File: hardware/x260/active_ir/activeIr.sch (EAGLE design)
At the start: 8 parts, among them Q1 MOSFET-N

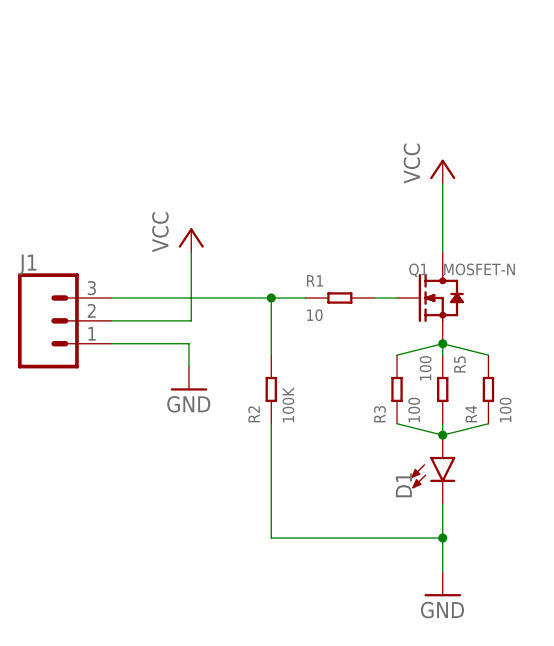
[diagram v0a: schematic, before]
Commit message: Initial simulation implementation
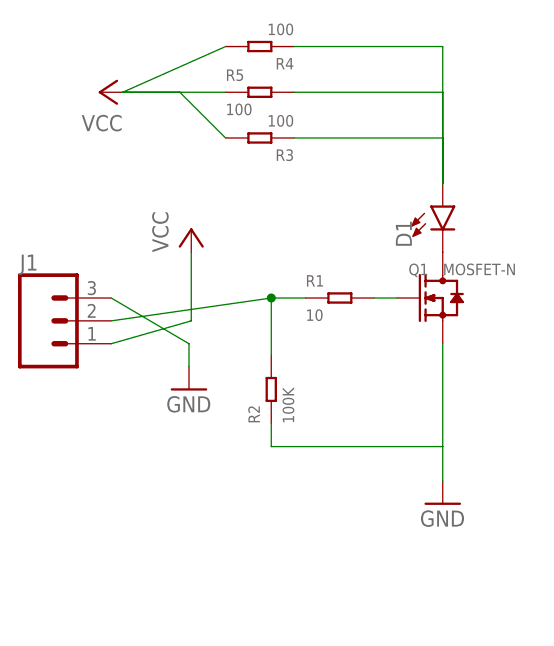
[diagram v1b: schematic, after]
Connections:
- net GND: now also J1.3, Q1.S; no longer D1.C, J1.1
- net N$1: now also D1.C, Q1.D; no longer Q1.S, R3.2, R4.2, R5.1
- net SIGNAL: now also J1.2; no longer J1.3
- net VCC: now also J1.1, R3.2, R4.2, R5.1; no longer J1.2, Q1.D
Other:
- moved on the sheet: D1, R3, R4, R5
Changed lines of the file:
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@@
 <instances>
 <instance part="Q1" gate="Q" x="53.34" y="45.72"/>
-<instance part="P+1" gate="VCC" x="53.34" y="60.96"/>
-<instance part="GND1" gate="1" x="53.34" y="12.7"/>
-<instance part="D1" gate="G$1" x="53.34" y="27.94"/>
+<instance part="P+1" gate="VCC" x="15.24" y="68.58" rot="R90"/>
+<instance part="GND1" gate="1" x="53.34" y="22.86"/>
+<instance part="D1" gate="G$1" x="53.34" y="55.88"/>
 <instance part="R2" gate="R" x="34.29" y="35.56" rot="R90"/>
 <instance part="R1" gate="R" x="41.91" y="45.72"/>
-<instance part="R3" gate="R" x="48.26" y="35.56" rot="R90"/>
+<instance part="R3" gate="R" x="33.02" y="63.5" rot="R180"/>
 <instance part="J1" gate="J$1" x="8.89" y="43.18"/>
 <instance part="P+2" gate="VCC" x="25.4" y="53.34"/>
 <instance part="GND2" gate="1" x="25.146" y="35.56"/>
-<instance part="R4" gate="R" x="58.42" y="35.56" rot="R90"/>
-<instance part="R5" gate="R" x="53.34" y="35.56" rot="R270"/>
+<instance part="R4" gate="R" x="33.02" y="73.66" rot="R180"/>
+<instance part="R5" gate="R" x="33.02" y="68.58"/>
 </instances>
 <busses>
@@
 <net name="VCC" class="0">
 <segment>
-<pinref part="Q1" gate="Q" pin="D"/>
-<pinref part="P+1" gate="VCC" pin="VCC"/>
-<wire x1="53.34" y1="58.42" x2="53.34" y2="50.8" width="0.1524" layer="91"/>
+<pinref part="J1" gate="J$1" pin="1"/>
+<pinref part="P+2" gate="VCC" pin="VCC"/>
+<wire x1="25.4" y1="50.8" x2="25.4" y2="43.18" width="0.1524" layer="91"/>
+<wire x1="25.4" y1="43.18" x2="16.51" y2="40.64" width="0.1524" layer="91"/>
 </segment>
 <segment>
-<pinref part="J1" gate="J$1" pin="2"/>
-<pinref part="P+2" gate="VCC" pin="VCC"/>
-<wire x1="25.4" y1="50.8" x2="25.4" y2="43.18" width="0.1524" layer="91"/>
-<wire x1="25.4" y1="43.18" x2="16.51" y2="43.18" width="0.1524" layer="91"/>
+<pinref part="R4" gate="R" pin="2"/>
+<pinref part="P+1" gate="VCC" pin="VCC"/>
+<wire x1="29.21" y1="73.66" x2="17.78" y2="68.58" width="0.1524" layer="91"/>
+<pinref part="R5" gate="R" pin="1"/>
+<wire x1="29.21" y1="68.58" x2="17.78" y2="68.58" width="0.1524" layer="91"/>
+<pinref part="R3" gate="R" pin="2"/>
+<wire x1="29.21" y1="63.5" x2="24.13" y2="68.58" width="0.1524" layer="91"/>
+<wire x1="24.13" y1="68.58" x2="17.78" y2="68.58" width="0.1524" layer="91"/>
 </segment>
 </net>
 <net name="GND" class="0">
 <segment>
-<pinref part="D1" gate="G$1" pin="C"/>
 <pinref part="GND1" gate="1" pin="GND"/>
-<wire x1="53.34" y1="15.24" x2="53.34" y2="19.05" width="0.1524" layer="91"/>
 <pinref part="R2" gate="R" pin="1"/>
-<wire x1="53.34" y1="19.05" x2="53.34" y2="22.86" width="0.1524" layer="91"/>
-<wire x1="34.29" y1="31.75" x2="34.29" y2="19.05" width="0.1524" layer="91"/>
-<wire x1="34.29" y1="19.05" x2="53.34" y2="19.05" width="0.1524" layer="91"/>
-<junction x="53.34" y="19.05"/>
+<wire x1="53.34" y1="25.4" x2="53.34" y2="29.21" width="0.1524" layer="91"/>
+<wire x1="34.29" y1="31.75" x2="34.29" y2="29.21" width="0.1524" layer="91"/>
+<wire x1="34.29" y1="29.21" x2="53.34" y2="29.21" width="0.1524" layer="91"/>
+<pinref part="Q1" gate="Q" pin="S"/>
+<wire x1="53.34" y1="40.64" x2="53.34" y2="29.21" width="0.1524" layer="91"/>
 </segment>
 <segment>
-<pinref part="J1" gate="J$1" pin="1"/>
+<pinref part="J1" gate="J$1" pin="3"/>
 <pinref part="GND2" gate="1" pin="GND"/>
 <wire x1="25.146" y1="38.1" x2="25.146" y2="40.64" width="0.1524" layer="91"/>
-<wire x1="25.146" y1="40.64" x2="16.51" y2="40.64" width="0.1524" layer="91"/>
-</segment>
-</net>
-<net name="N$1" class="0">
-<segment>
-<pinref part="Q1" gate="Q" pin="S"/>
-<pinref part="R3" gate="R" pin="2"/>
-<wire x1="48.26" y1="39.37" x2="53.34" y2="40.64" width="0.1524" layer="91"/>
-<pinref part="R4" gate="R" pin="2"/>
-<wire x1="58.42" y1="39.37" x2="53.34" y2="40.64" width="0.1524" layer="91"/>
-<junction x="53.34" y="40.64"/>
-<pinref part="R5" gate="R" pin="1"/>
-<wire x1="53.34" y1="39.37" x2="53.34" y2="40.64" width="0.1524" layer="91"/>
+<wire x1="25.146" y1="40.64" x2="16.51" y2="45.72" width="0.1524" layer="91"/>
 </segment>
 </net>
@@
 <pinref part="R3" gate="R" pin="1"/>
 <pinref part="D1" gate="G$1" pin="A"/>
-<wire x1="53.34" y1="30.48" x2="48.26" y2="31.75" width="0.1524" layer="91"/>
+<wire x1="53.34" y1="58.42" x2="53.34" y2="63.5" width="0.1524" layer="91"/>
+<wire x1="53.34" y1="63.5" x2="36.83" y2="63.5" width="0.1524" layer="91"/>
 <pinref part="R4" gate="R" pin="1"/>
-<wire x1="58.42" y1="31.75" x2="53.34" y2="30.48" width="0.1524" layer="91"/>
-<junction x="53.34" y="30.48"/>
+<wire x1="36.83" y1="73.66" x2="53.34" y2="73.66" width="0.1524" layer="91"/>
+<wire x1="53.34" y1="73.66" x2="53.34" y2="58.42" width="0.1524" layer="91"/>
 <pinref part="R5" gate="R" pin="2"/>
-<wire x1="53.34" y1="31.75" x2="53.34" y2="30.48" width="0.1524" layer="91"/>
+<wire x1="36.83" y1="68.58" x2="53.34" y2="68.58" width="0.1524" layer="91"/>
+<wire x1="53.34" y1="68.58" x2="53.34" y2="58.42" width="0.1524" layer="91"/>
 </segment>
 </net>
@@
 <segment>
 <pinref part="R1" gate="R" pin="1"/>
-<pinref part="J1" gate="J$1" pin="3"/>
-<wire x1="16.51" y1="45.72" x2="34.29" y2="45.72" width="0.1524" layer="91"/>
+<pinref part="J1" gate="J$1" pin="2"/>
+<wire x1="16.51" y1="43.18" x2="34.29" y2="45.72" width="0.1524" layer="91"/>
 <pinref part="R2" gate="R" pin="2"/>
 <wire x1="34.29" y1="45.72" x2="38.1" y2="45.72" width="0.1524" layer="91"/>
@@
 </segment>
 </net>
+<net name="N$1" class="0">
+<segment>
+<pinref part="Q1" gate="Q" pin="D"/>
+<pinref part="D1" gate="G$1" pin="C"/>
+</segment>
+</net>
